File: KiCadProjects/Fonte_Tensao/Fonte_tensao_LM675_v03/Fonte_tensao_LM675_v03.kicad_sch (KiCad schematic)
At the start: 32 parts, among them J1 Barrel_Jack, J2 sinais analogicos, J3 comunicacao / sinais digitais, J4 tensoes, U1 L7809, U2 LM7909_TO220, U3 LM675, U4 L7805, U5 L7905, U6 LM1117T-3.3

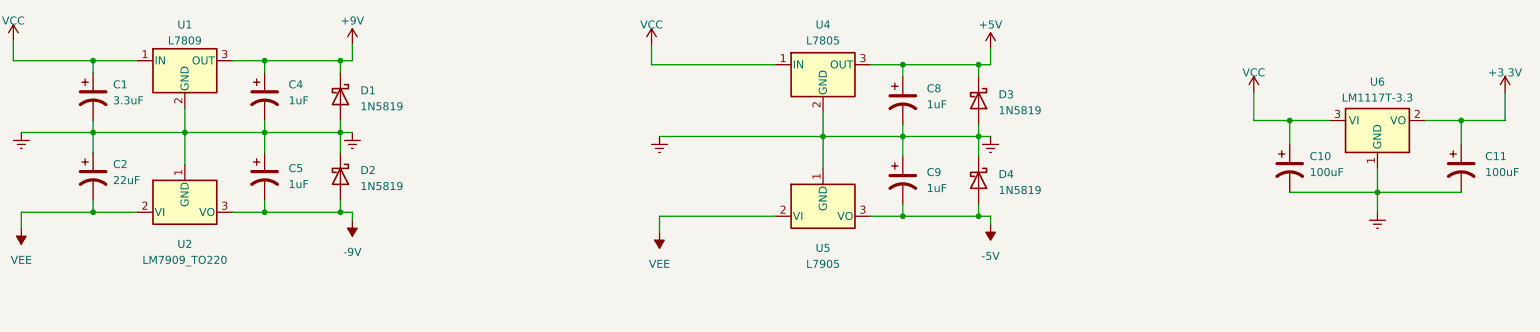
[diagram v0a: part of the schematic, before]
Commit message: revisar alteracoes fonte tensao v3
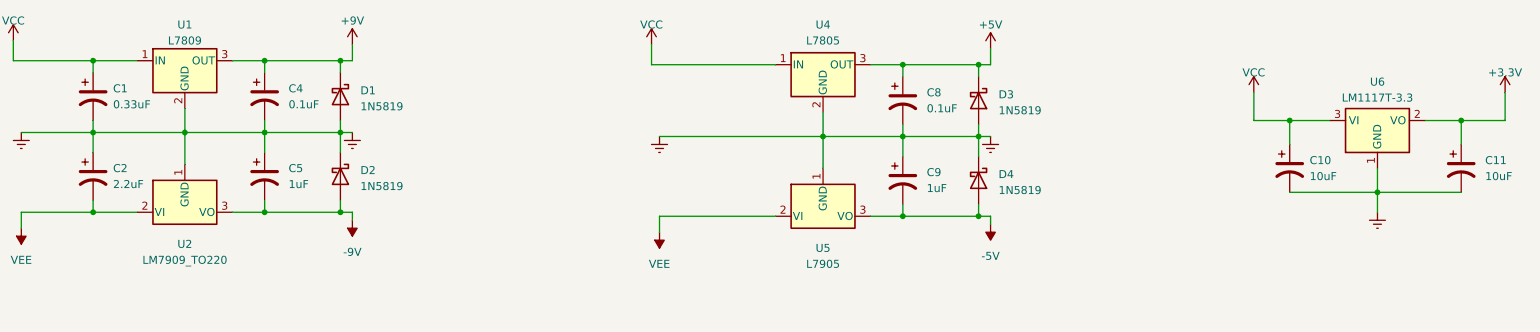
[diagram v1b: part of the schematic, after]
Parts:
- C1: value 3.3uF -> 0.33uF
- C10, C11: value 100uF -> 10uF
- C2: value 22uF -> 2.2uF
- C4, C8: value 1uF -> 0.1uF
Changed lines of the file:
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@@
     (company "EITduino")
     (comment 1 "Autor: Gustavo Pinheiro")
+    (comment 2 "reguladores: usar capacitores de tantalo")
     (comment 3 "Chave gangorra kcd1 no lugar do botao para acionamento")
   )
@@
   (symbol (lib_id "Device:C_Polarized_US") (at 72.39 38.1 0) (unit 1)
     (in_bom yes) (on_board yes) (dnp no) (fields_autoplaced)
-    (property "Reference" "C4" (at 76.2 36.195 0)
-      (effects (font (size 1.27 1.27)) (justify left))
-    )
-    (property "Value" "1uF" (at 76.2 38.735 0)
+    (property "Reference" "C4" (at 76.2 36.83 0)
+      (effects (font (size 1.27 1.27)) (justify left))
+    )
+    (property "Value" "0.1uF" (at 76.2 39.37 0)
       (effects (font (size 1.27 1.27)) (justify left))
     )
@@
   (symbol (lib_id "Device:C_Polarized_US") (at 235.585 49.53 0) (unit 1)
     (in_bom yes) (on_board yes) (dnp no) (fields_autoplaced)
-    (property "Reference" "C10" (at 238.76 47.625 0)
-      (effects (font (size 1.27 1.27)) (justify left))
-    )
-    (property "Value" "100uF" (at 238.76 50.165 0)
+    (property "Reference" "C10" (at 238.76 48.26 0)
+      (effects (font (size 1.27 1.27)) (justify left))
+    )
+    (property "Value" "10uF" (at 238.76 50.8 0)
       (effects (font (size 1.27 1.27)) (justify left))
     )
@@
   (symbol (lib_id "Device:C_Polarized_US") (at 45.085 50.8 0) (unit 1)
     (in_bom yes) (on_board yes) (dnp no) (fields_autoplaced)
-    (property "Reference" "C2" (at 48.26 48.895 0)
-      (effects (font (size 1.27 1.27)) (justify left))
-    )
-    (property "Value" "22uF" (at 48.26 51.435 0)
+    (property "Reference" "C2" (at 48.26 49.53 0)
+      (effects (font (size 1.27 1.27)) (justify left))
+    )
+    (property "Value" "2.2uF" (at 48.26 52.07 0)
       (effects (font (size 1.27 1.27)) (justify left))
     )
@@
   (symbol (lib_id "Device:C_Polarized_US") (at 45.085 38.1 0) (unit 1)
     (in_bom yes) (on_board yes) (dnp no) (fields_autoplaced)
-    (property "Reference" "C1" (at 48.26 36.195 0)
-      (effects (font (size 1.27 1.27)) (justify left))
-    )
-    (property "Value" "3.3uF" (at 48.26 38.735 0)
+    (property "Reference" "C1" (at 48.26 36.83 0)
+      (effects (font (size 1.27 1.27)) (justify left))
+    )
+    (property "Value" "0.33uF" (at 48.26 39.37 0)
       (effects (font (size 1.27 1.27)) (justify left))
     )
@@
   (symbol (lib_id "Device:C_Polarized_US") (at 262.89 49.53 0) (unit 1)
     (in_bom yes) (on_board yes) (dnp no) (fields_autoplaced)
-    (property "Reference" "C11" (at 266.7 47.625 0)
-      (effects (font (size 1.27 1.27)) (justify left))
-    )
-    (property "Value" "100uF" (at 266.7 50.165 0)
+    (property "Reference" "C11" (at 266.7 48.26 0)
+      (effects (font (size 1.27 1.27)) (justify left))
+    )
+    (property "Value" "10uF" (at 266.7 50.8 0)
       (effects (font (size 1.27 1.27)) (justify left))
     )
@@
   (symbol (lib_id "Device:C_Polarized_US") (at 173.99 38.735 0) (unit 1)
     (in_bom yes) (on_board yes) (dnp no) (fields_autoplaced)
-    (property "Reference" "C8" (at 177.8 36.83 0)
-      (effects (font (size 1.27 1.27)) (justify left))
-    )
-    (property "Value" "1uF" (at 177.8 39.37 0)
-      (effects (font (size 1.27 1.27)) (justify left))
-    )
+    (property "Reference" "C8" (at 177.8 37.465 0)
+      (effects (font (size 1.27 1.27)) (justify left))
+    )
+    (property "Value" "0.1uF" (at 177.8 40.005 0)
+      (effects (font (size 1.27 1.27)) (justify left))
+    )
